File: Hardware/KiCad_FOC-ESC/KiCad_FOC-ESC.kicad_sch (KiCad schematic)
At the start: 19 parts, among them J2 Prog, U1 STM32G473RCTx, U802 ZLDO1117Q

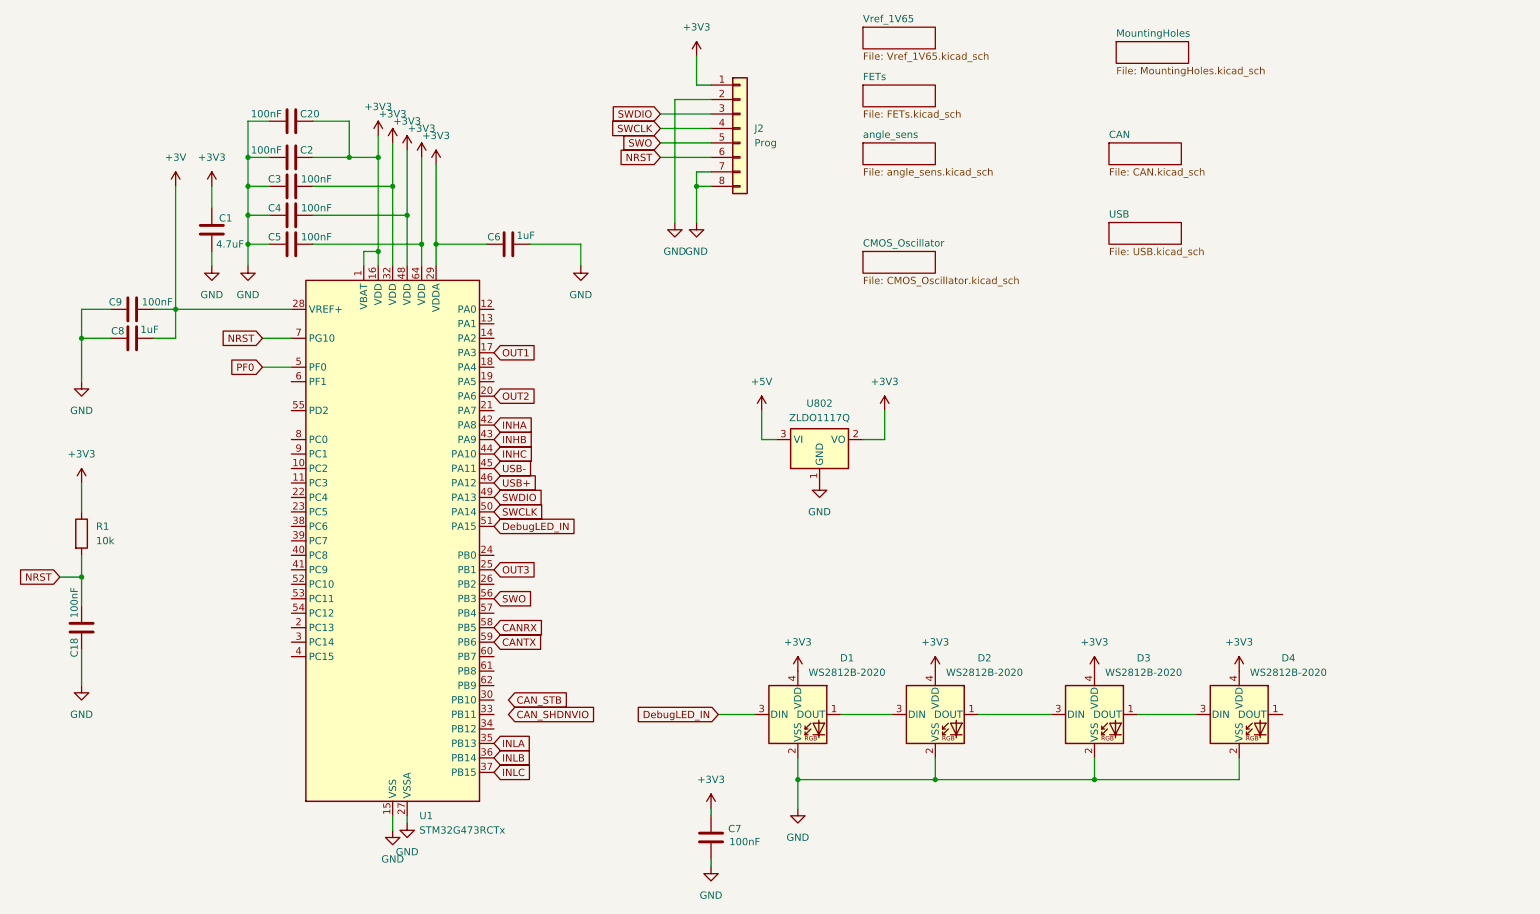
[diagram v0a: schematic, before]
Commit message: added:ferrite bead
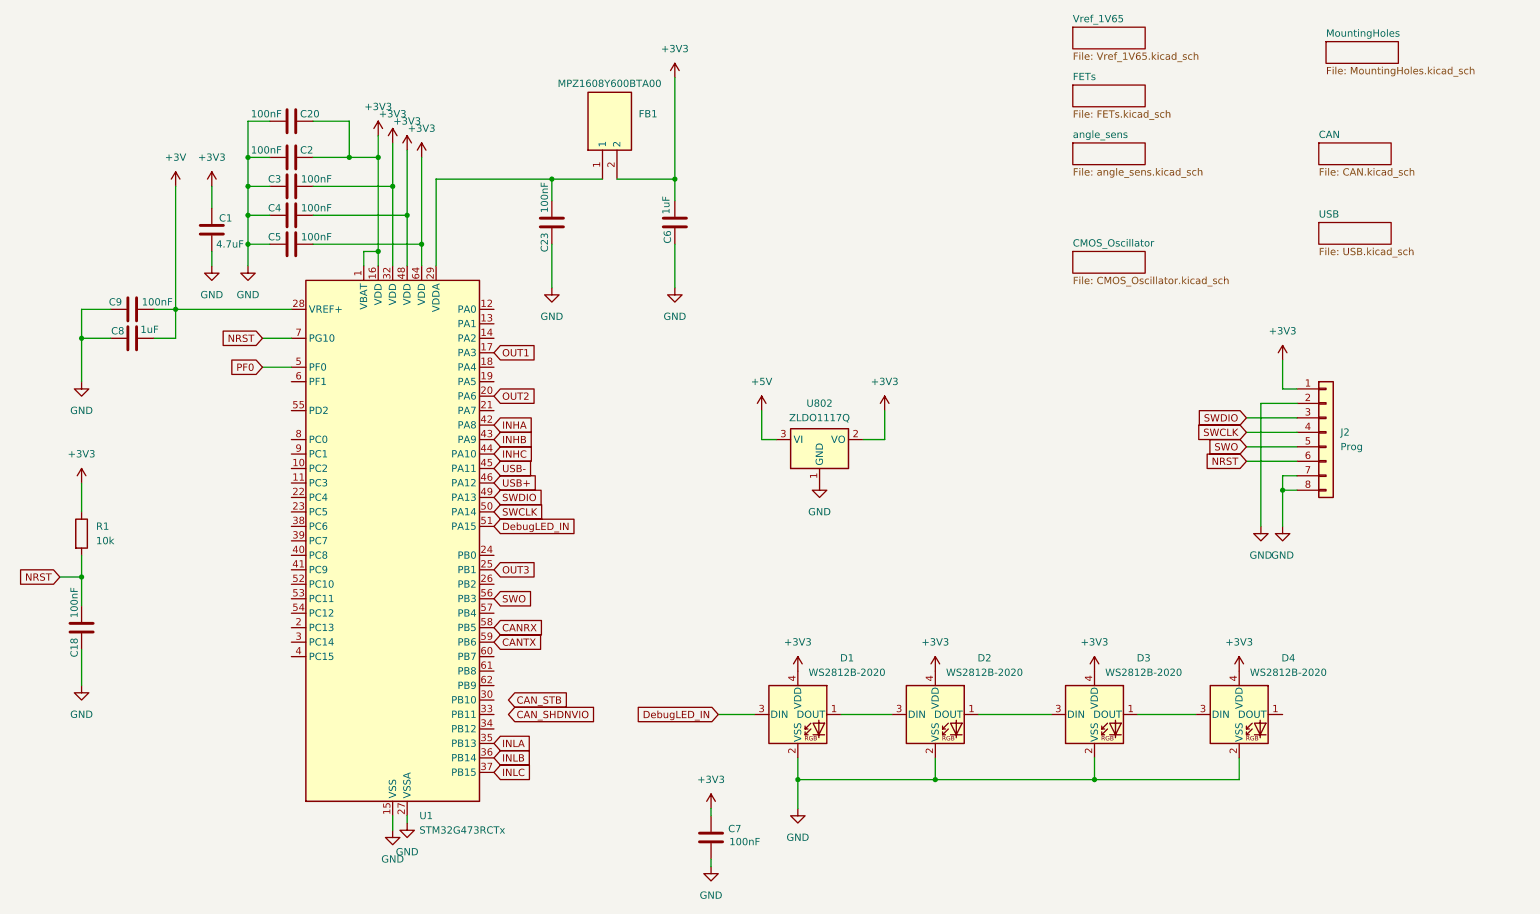
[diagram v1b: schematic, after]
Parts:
- added C23: 100nF, Capacitor_SMD:C_0402_1005Metric, symbol Device:C
- added FB1: MPZ1608Y600BTA00, BEADC1608X95N, symbol SamacSys_Parts:MPZ1608Y600BTA00
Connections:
- net +3V3: now also C6.2, FB1.2; no longer C6.1, U1.29 (VDDA)
- net GND: now also C6.1, C23.1; no longer C6.2
- new net: C23.2, FB1.1, U1.29 (VDDA)
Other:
- moved on the sheet: C6, J2
